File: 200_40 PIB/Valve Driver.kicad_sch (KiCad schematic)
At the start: 20 parts, among them J12 532610671, Q10 IRF7832, U1 LT3065EDDPBF, U2 MIC4424YM, U3 MIC4424YM

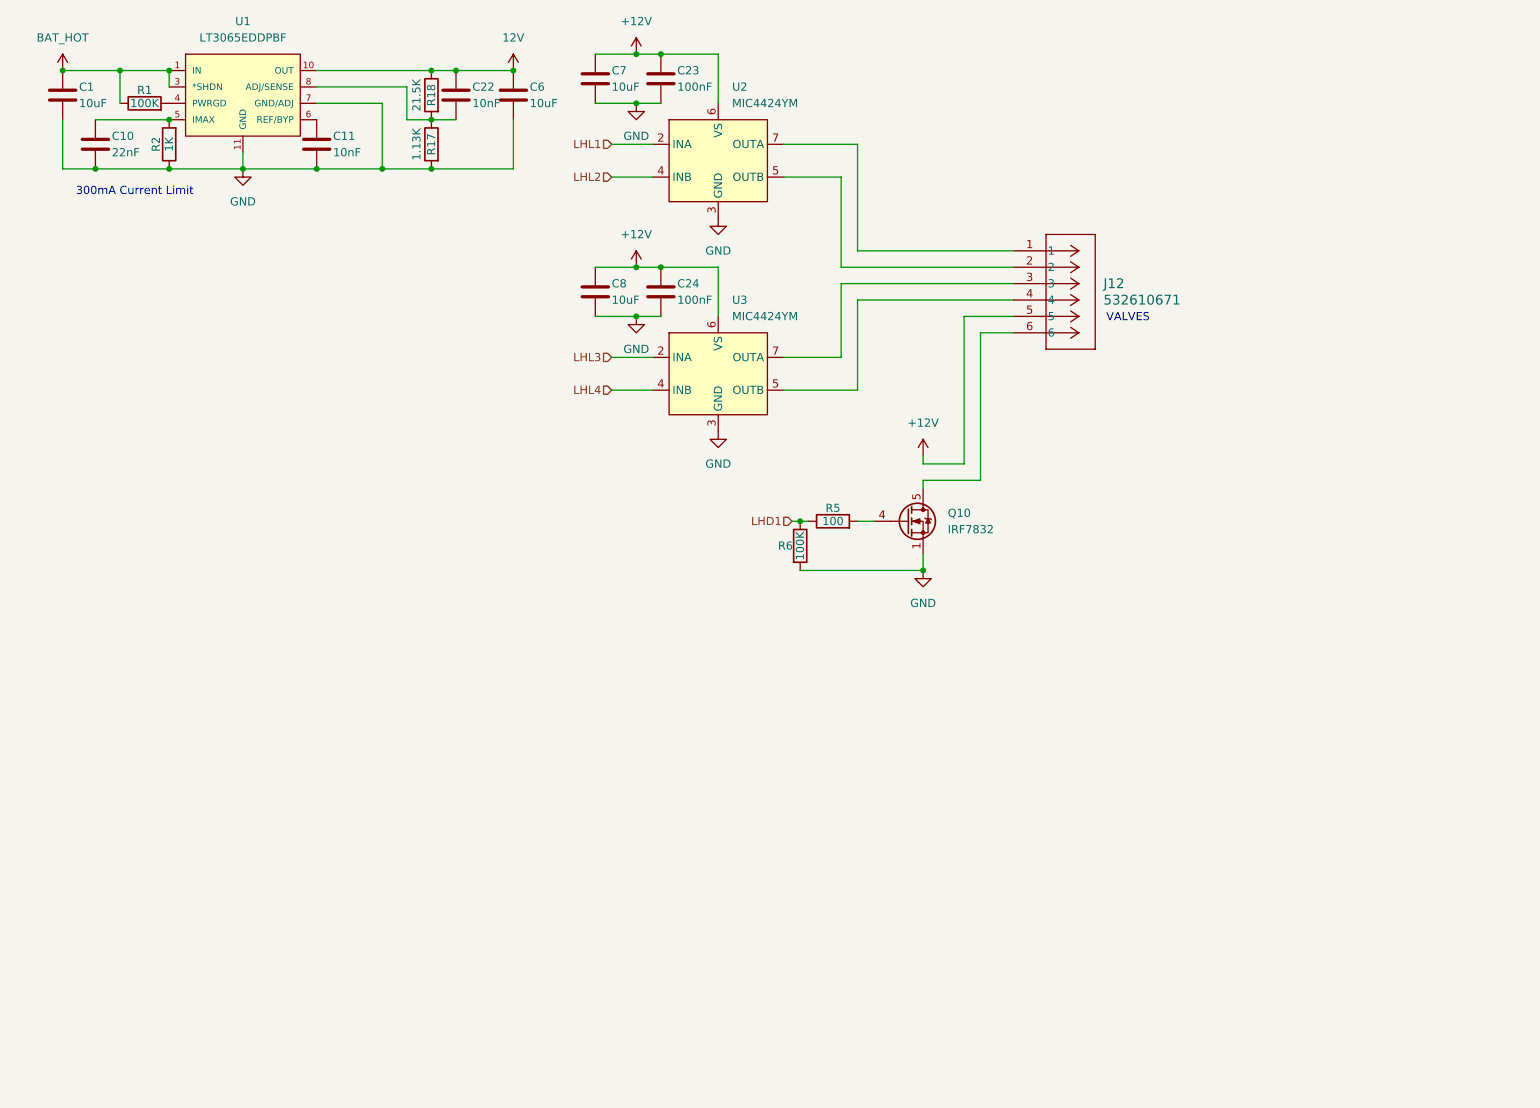
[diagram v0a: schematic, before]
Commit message: pib work
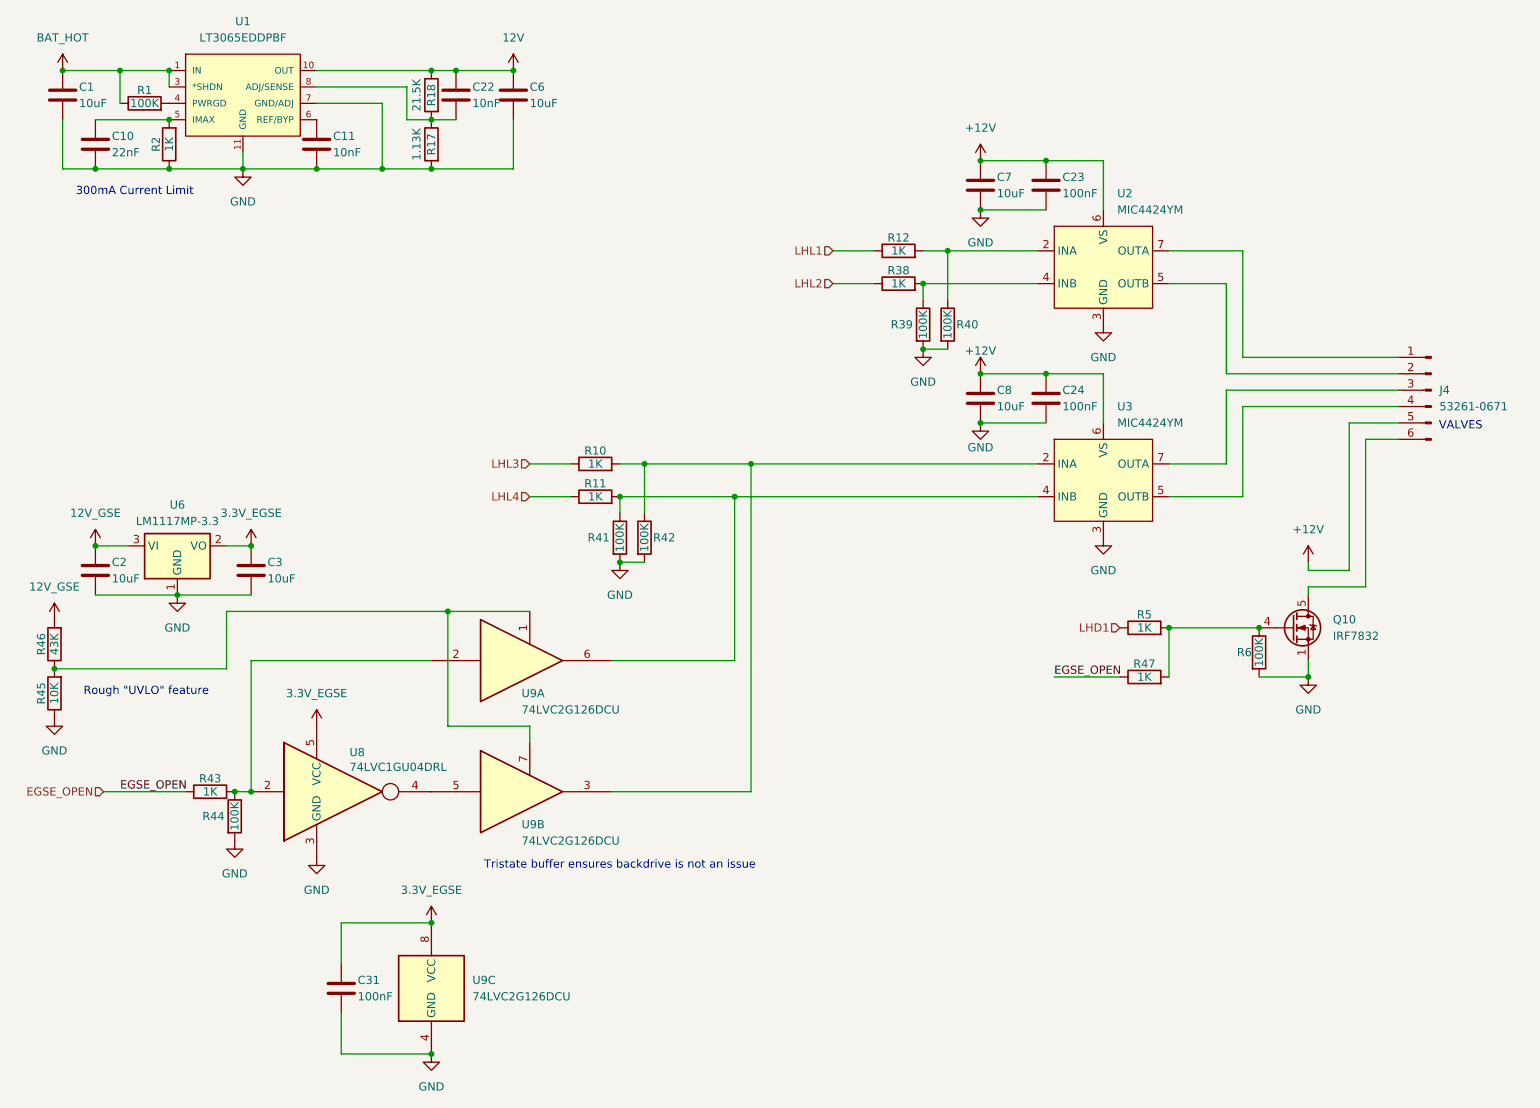
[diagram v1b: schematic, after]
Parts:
- removed J12: 532610671, CONN_532610001-SD_06_MOL, symbol 0_PAY_Symbol_Library:532610671
- added C2, C3: 10uF, Capacitor_SMD:C_0805_2012Metric, symbol Device:C
- added C31: 100nF, Capacitor_SMD:C_0402_1005Metric, symbol Device:C
- added J4: 53261-0671, Connector_Molex:Molex_PicoBlade_53261-0671_1x06-1MP_P1.25mm_Horizontal, symbol Connector:Conn_01x06_Pin
- added R10, R11, R12, R38, R43, R47: 1K, Resistor_SMD:R_0402_1005Metric, symbol Device:R
- added R39, R40, R41, R42, R44: 100K, symbol Device:R
- added R45: 10K, Capacitor_SMD:C_0603_1608Metric, symbol Device:R
- added R46: 43K, Capacitor_SMD:C_0603_1608Metric, symbol Device:R
- added U6: LM1117MP-3.3, Package_TO_SOT_SMD:SOT-223-3_TabPin2, symbol Regulator_Linear:LM1117MP-3.3
- added U8: 74LVC1GU04DRL, Package_TO_SOT_SMD:SOT-553, symbol 74xGxx:74LVC1GU04DRL
- added U9: 74LVC2G126DCU, symbol 74xGxx:74LVC2G126
- R5: value 100 -> 1K
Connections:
- net +12V: now also J4.5 (Pin_5)
- net GND: now also C2.2, C3.2, C31.2, R39.2, R40.2, R41.2, R42.2, R44.2, R45.1, U6.1 (GND), U8.3 (GND), U9.4 (GND)
- net LHD1: no longer R6.1
- net LHL1: now also R12.1; no longer U2.2 (INA)
- net LHL2: now also R38.1; no longer U2.4 (INB)
- net LHL3: now also R10.1; no longer U3.2 (INA)
- net LHL4: now also R11.1; no longer U3.4 (INB)
- net at U2.7 (OUTA): now also J4.1 (Pin_1)
- net at U2.5 (OUTB): now also J4.2 (Pin_2)
- net at U3.7 (OUTA): now also J4.3 (Pin_3)
- net at U3.5 (OUTB): now also J4.4 (Pin_4)
- net at Q10.5 (D), Q10.6 (D), Q10.7 (D)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: now also J4.6 (Pin_6)
- net at Q10.4 (G), R5.2: now also R6.1, R47.2
- new net: R10.2, R42.1, U3.2 (INA), U9.3
- new net: U8.4, U9.5
- new net: R45.2, R46.1, U9.1, U9.7
- new net: R12.2, R40.1, U2.2 (INA)
- new net: R43.2, R44.1, U8.2, U9.2
- new net: R11.2, R41.1, U3.4 (INB), U9.6
- new net: R38.2, R39.1, U2.4 (INB)
- new net 12V_GSE: C2.1, R46.2, U6.3 (VI)
- new net 3.3V_EGSE: C3.1, C31.1, U6.2 (VO), U8.5 (VCC), U9.8 (VCC)
- new net EGSE_OPEN: R43.1, R47.1
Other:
- note added: "Rough "UVLO" feature"
- note added: "Tristate buffer ensures backdrive is not an issue"
- moved on the sheet: C23, C24, C7, C8, Q10, R5, R6, U2, U3
